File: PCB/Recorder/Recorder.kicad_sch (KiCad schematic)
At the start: 53 parts, among them J1 Battery, J2 Reset, J3 TC2030-USB-NL-DS, J4 TF_PUSH, J5 USB-C-Socket-H, Q2 CJ2301, SW1 SW_Push, U1 R, U2 ESP32-S3-MINI-1, U2 L, U3 TP4054, U4 ME6211C33M5G-N, U5 MAX98357A

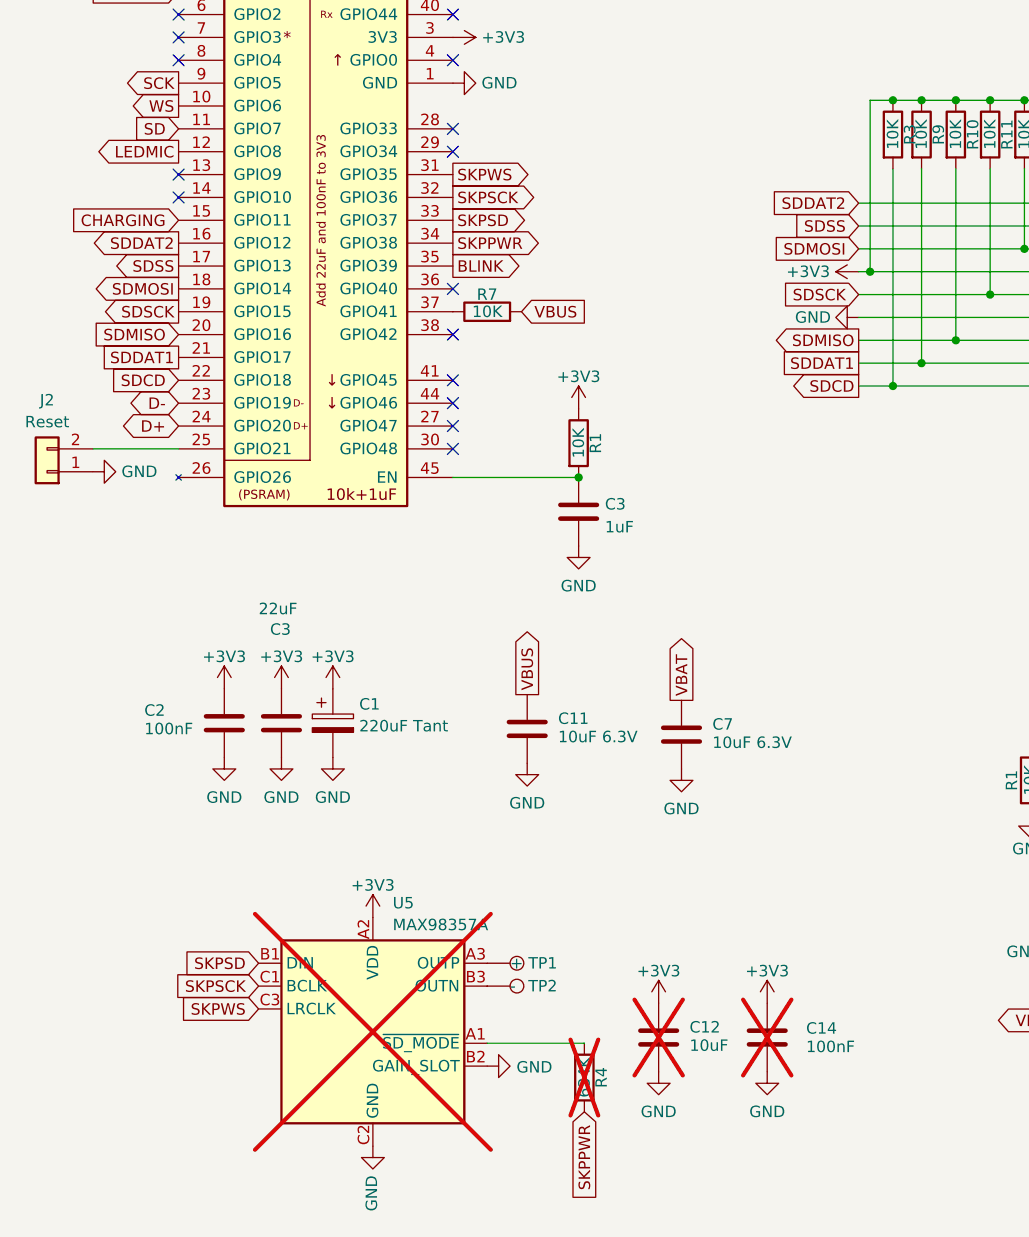
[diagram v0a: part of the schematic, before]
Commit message: Tidy
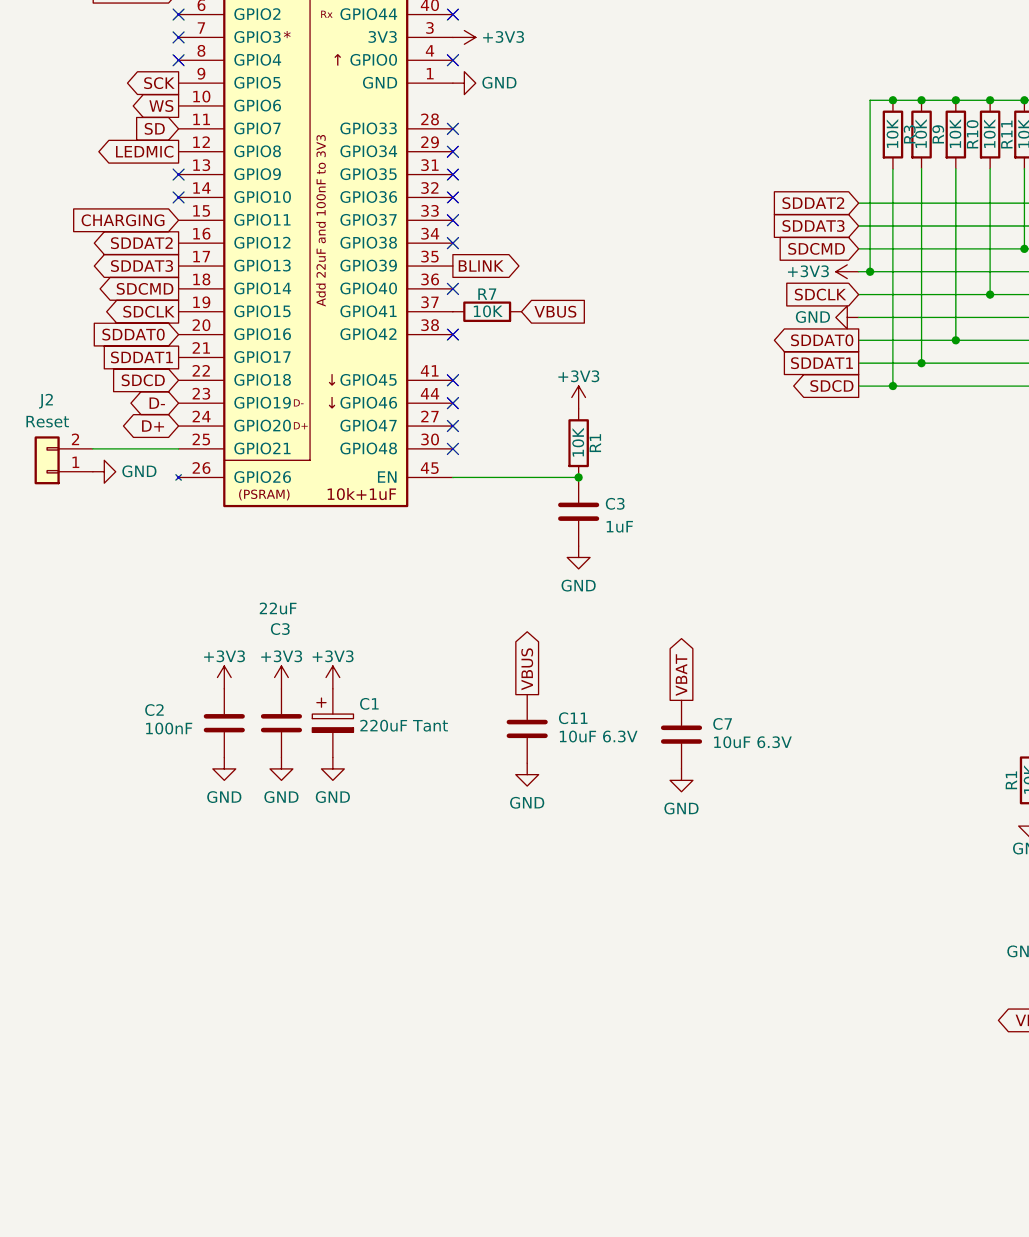
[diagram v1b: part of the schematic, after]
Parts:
- removed C12: 10uF, RevK:C_0402, symbol Device:C
- removed C14: 100nF, RevK:C_0402, symbol Device:C
- removed R4: 634K, RevK:R_0402, symbol Device:R
- removed TP1: +, RevK:SolderPadSmall, symbol Connector:TestPoint
- removed TP2: -, RevK:SolderPadSmall, symbol Connector:TestPoint
- removed U5: MAX98357A, RevK:WLP-1.437mmx1.347mm-0.21mm-ball, symbol RevK:MAX98357A
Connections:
- net SDMISO renamed SDDAT0
- net SDMOSI renamed SDCMD
- net SDSCK renamed SDCLK
- net SDSS renamed SDDAT3
- net SKPPWR: no longer names the net of U2.34 (GPIO38)
- net SKPSCK: no longer names the net of U2.32 (GPIO36)
- net SKPSD: no longer names the net of U2.33 (GPIO37)
- net SKPWS: no longer names the net of U2.31 (GPIO35)
- no-connect marks 18 -> 22
